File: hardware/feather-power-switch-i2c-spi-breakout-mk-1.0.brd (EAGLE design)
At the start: 22.9 x 17.8 mm, 13 parts, among them U1_ ROTARY_ENCODER_SWITCH, U2 Tiny85

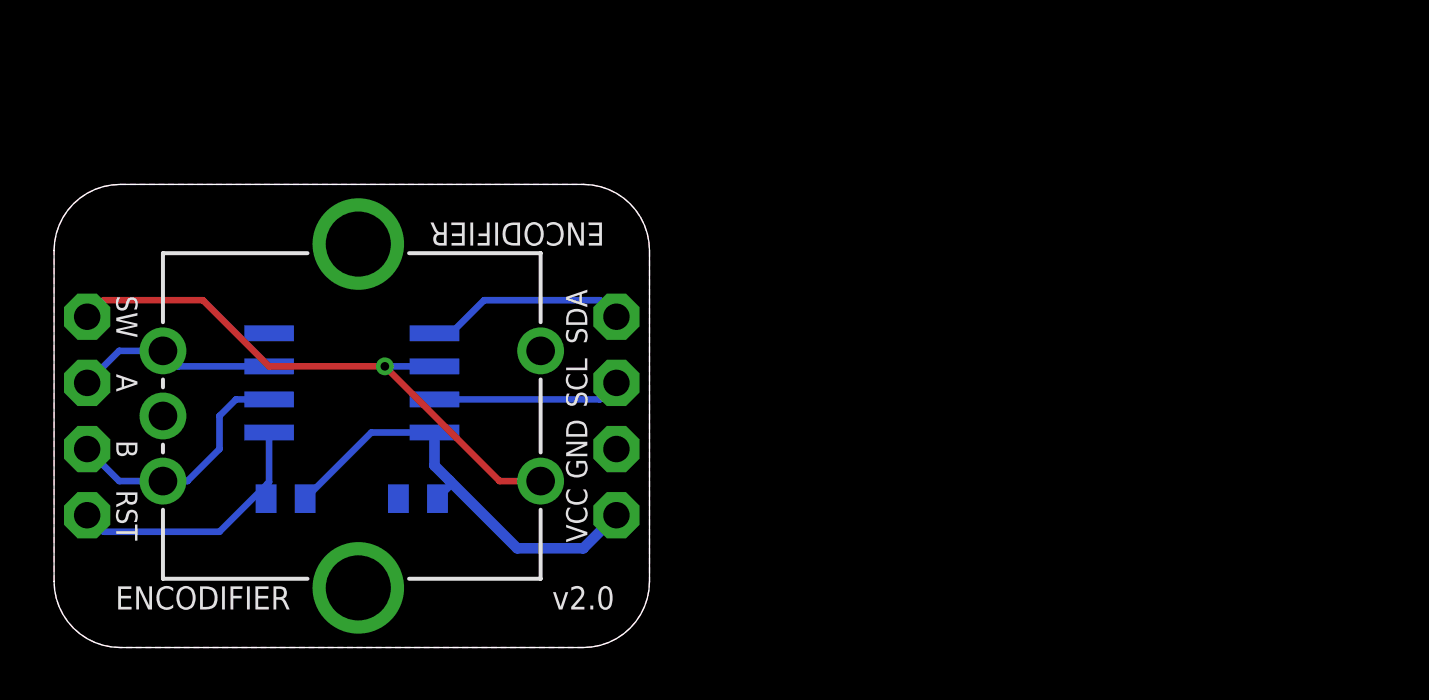
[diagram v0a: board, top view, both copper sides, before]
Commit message: have some boards, dawg
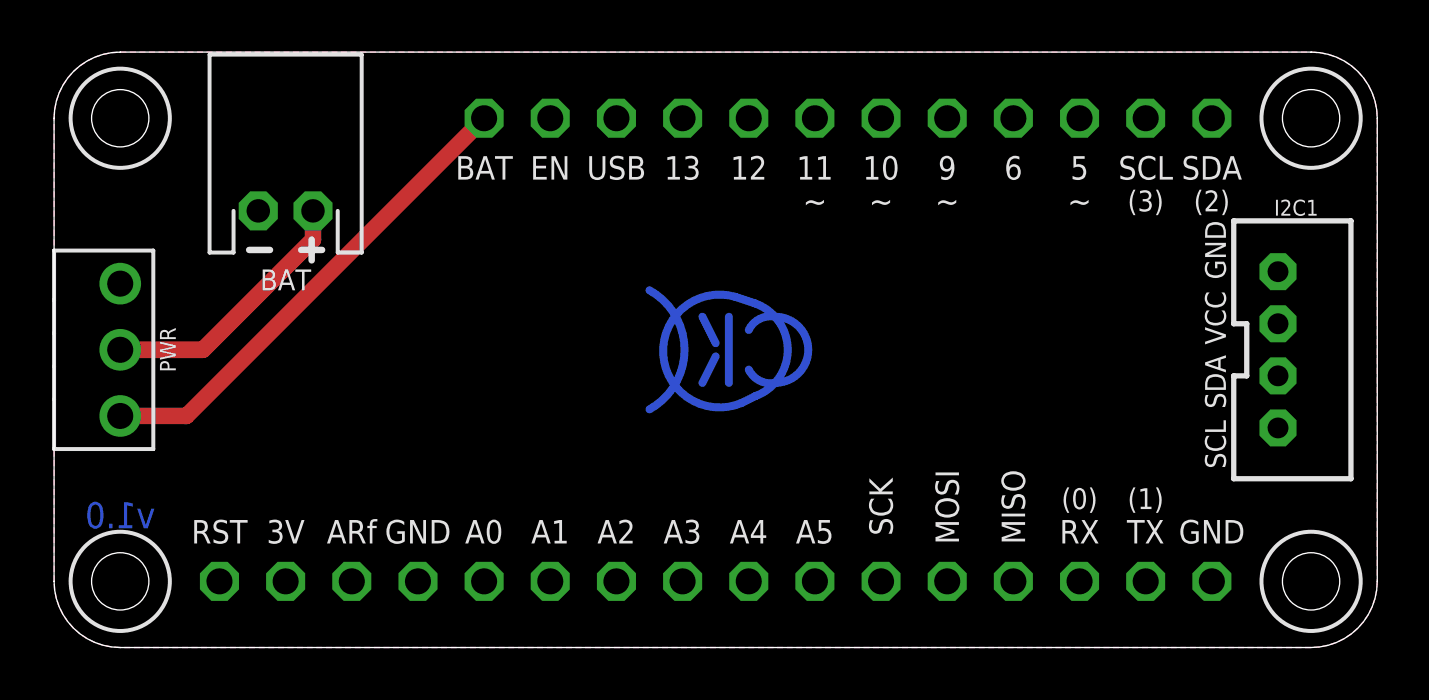
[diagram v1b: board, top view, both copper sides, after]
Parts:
- removed A, B, GND, RST, SCL, SDA, SW, VCC: M01PTH-1MM, a_parts:1X01-1MM-NS
- removed C1: 100n, a_parts:C0603-TIGHTER
- removed R1: 10k, a_parts:R0603-TIGHTER
- removed U1_: ROTARY_ENCODER_SWITCH, a_parts:ROTARY_ENCODER_SWITCH
- removed U2: Tiny85, a_parts:SO08-EIAJ
- added BAT: M02JST-PTH-RA-R+, a_parts:JST-2-PH-RA-PTH-R+
- added I2C1: M04-I2CJST-4-PH-VERT-CENTERED-I2C, a_parts:JST-4-PH-VERT-PTH-CENTERED-I2C
- added PWR: SWITCH-SPDTPTH-RA-2.54MM, a_parts:SPDT-RA-2.54MM
- added U$1: (no value), a_parts:COW_SMALL_METAL_NOTEXT
- added U1: ADAFRUIT_FEATHER_SHIELD, a_parts:ADAFRUIT_FEATHER
- FRAME1: device A_butts:DUMMY -> a_parts:DUMMY
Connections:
- removed net A: A.1, U1_.A, U2.3
- removed net B: B.1, U1_.B, U2.2
- removed net MOSI/SDA: SDA.1, U2.5
- removed net RST: R1.1, RST.1, U2.1
- removed net SCK/SCL: SCL.1, U2.7
- removed net SW: SW.1, U1_.SW1, U2.6
- removed net VCC: C1.1, R1.2, U2.8, VCC.1
- new net 3V: I2C1.2, U1.3V
- new net N$1: BAT.2, PWR.2
- new net SCL: I2C1.4, U1.SCL
- new net SDA: I2C1.3, U1.SDA
- new net VBAT: PWR.3, U1.BAT
- net GND: now also BAT.1, I2C1.1, U1.GND@0, U1.GND@1; no longer C1.2, GND.1, U1_.C, U1_.SW2, U2.4
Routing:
- net SW: track 22.5 -> 0.00 mm, vias 1 -> 0
- net VBAT: track 0.00 -> 18.7 mm
- net VCC: track 17.0 -> 0.00 mm
- net RST: track 10.5 -> 0.00 mm
- net N$1: track 0.00 -> 10.3 mm
- net B: track 9.54 -> 0.00 mm
- net MOSI/SDA: track 7.77 -> 0.00 mm
- net A: track 7.74 -> 0.00 mm
- net SCK/SCL: track 7.25 -> 0.00 mm
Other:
- board size 22.9 x 17.8 mm -> 50.8 x 22.9 mm
- board text removed: "A"
- board text removed: "B"
- board text removed: "C"
- board text removed: "COM"
- board text removed: "ENCODIFIER"
- board text removed: "SW"
